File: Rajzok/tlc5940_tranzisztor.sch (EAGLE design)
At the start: 17 parts, among them Q1 TP0602N2, Q2 TP0602N2, Q3 SUP75N06-08, Q4 SUP75N06-08

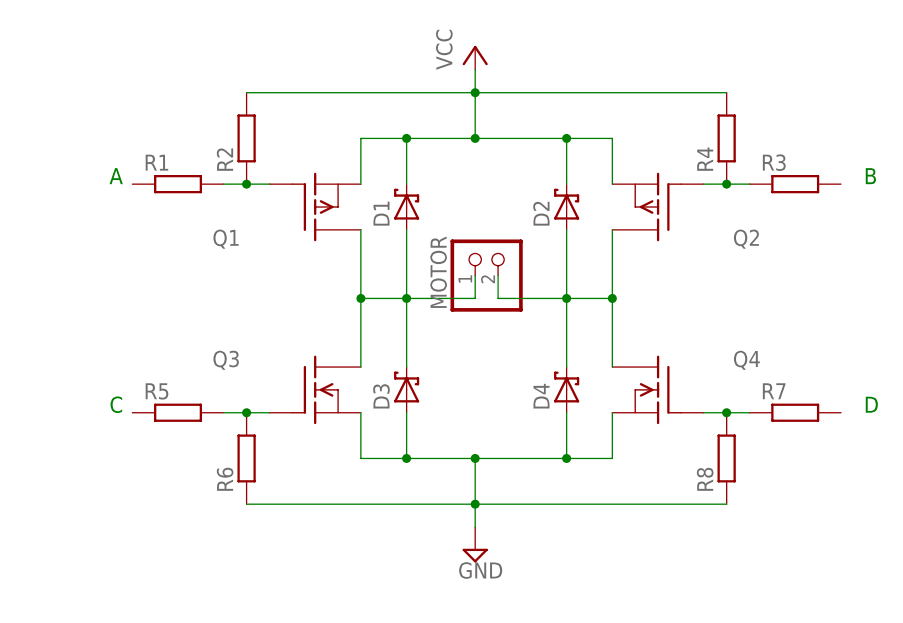
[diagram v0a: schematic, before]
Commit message: Rajzok 2017
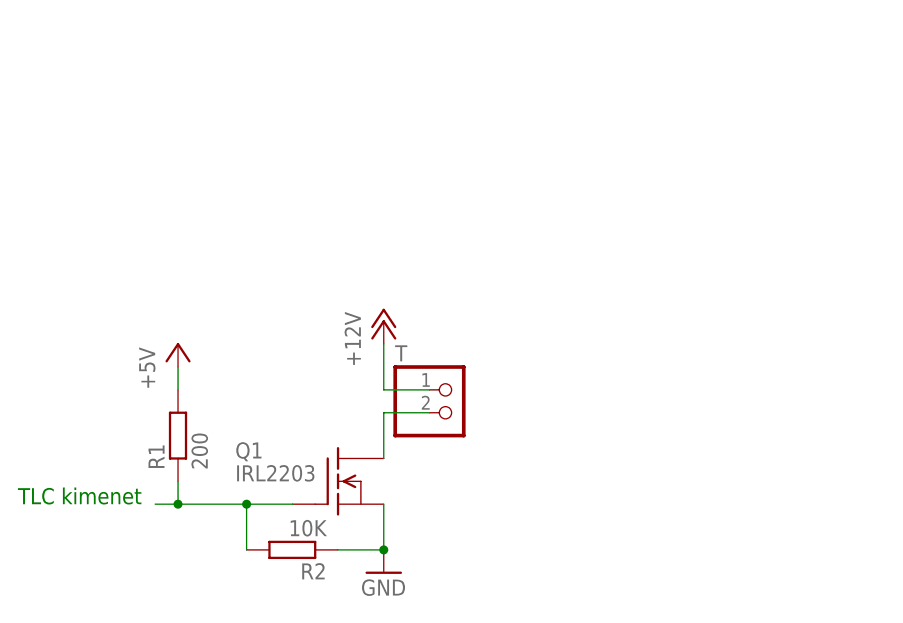
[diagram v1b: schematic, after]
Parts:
- removed D1, D2, D3, D4: 1N6267A, diode:1N6267A
- removed MOTOR: (no value), pinhead:PINHD-1X2
- removed Q2: TP0602N2, transistor-fet:TP0602N2
- removed Q3, Q4: SUP75N06-08, transistor-fet:SUP75N06-08
- removed R3, R4, R5, R6, R7, R8: (no value), rcl:R-EU_0204/7
- added T: (no value), pinhead:PINHD-1X2
- Q1: value TP0602N2 -> IRL2203; device transistor-fet:TP0602N2 -> transistor-fet:BUZ10
- R1: value (none) -> 200; device rcl:R-EU_0204/7 -> rcl:R-EU_0207/10
- R2: value (none) -> 10K; device rcl:R-EU_0204/7 -> rcl:R-EU_0207/10
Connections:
- removed net N$3: Q2.G, R3.1, R4.1
- removed net N$4: Q3.G, R5.2, R6.2
- removed net N$5: Q4.G, R7.1, R8.2
- removed net N$9: D1.A, D3.C, MOTOR.1, Q1.D, Q3.D
- removed net VCC: D1.C, D2.C, Q1.S, Q2.S, R2.2, R4.2
- new net +12V: T.1
- new net +5V: R1.2
- net GND: now also Q1.S, R2.1; no longer D3.A, D4.A, Q3.S, Q4.S, R6.1, R8.1
- net N$1: now also R1.1, R2.2; no longer R1.2, R2.1
- net N$2: now also Q1.D, T.2; no longer D2.A, D4.C, MOTOR.2, Q2.D, Q4.D
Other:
- note added: "TLC kimenet"
- note removed: "A"
- note removed: "B"
- note removed: "C"
- note removed: "D"
- moved on the sheet: Q1, R1, R2
